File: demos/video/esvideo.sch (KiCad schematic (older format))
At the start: 29 parts, among them U8 BT253, U9 BT473

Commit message: Update demos
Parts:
- C32, C33, C34, C35, C36, C37, C39, C40, C41: symbol C -> video_schlib:C
- C42, C51, C52: symbol CP -> video_schlib:CP
- L5: symbol INDUCTOR -> video_schlib:INDUCTOR
- R15, R22, R23, R24, R36, R37, R38, R42, R43, R44, R45, R46, R47, R8: symbol R -> video_schlib:R
- U8: symbol BT253 -> video_schlib:BT253
- U9: symbol BT473 -> video_schlib:BT473
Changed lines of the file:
@@
-EESchema Schematic File Version 2
-LIBS:video_schlib
-LIBS:power
+EESchema Schematic File Version 4
 LIBS:video-cache
 EELAYER 26 0
@@
 PCA0
 $Comp
-L GND #PWR0162
+L video_schlib:GND #PWR0162
 U 1 1 33A566EB
 P 9300 7800
@@
 Connection ~ 4350 3100
 $Comp
-L GND #PWR0163
+L video_schlib:GND #PWR0163
 U 1 1 3392D11C
 P 4350 4200
@@
 RED_IN
 $Comp
-L GND #PWR0164
+L video_schlib:GND #PWR0164
 U 1 1 335F5DFC
 P 12050 5050
@@
 $EndComp
 $Comp
-L C C32
+L video_schlib:C C32
 U 1 1 335F5DF2
 P 11800 5050
@@
 	6650 4600 6550 4600
 $Comp
-L GND #GND0165
+L video_schlib:GND #GND0165
 U 1 1 A458682C
 P 12850 4250
@@
 $EndComp
 $Comp
-L R R8
+L video_schlib:R R8
 U 1 1 A4586827
 P 12550 4250
@@
 PCA[0..2]
 $Comp
-L GND #GND0166
+L video_schlib:GND #GND0166
 U 1 1 32FA0485
 P 5650 8250
@@
 	11350 3650 13450 3650
 $Comp
-L GND #GND0167
+L video_schlib:GND #GND0167
 U 1 1 32F9F3E8
 P 10450 8250
@@
 RDCAD-
 $Comp
-L BT473 U9
+L video_schlib:BT473 U9
 U 1 1 32F9E902
 P 10350 5450
@@
 $EndComp
 $Comp
-L BT253 U8
+L video_schlib:BT253 U8
 U 1 1 32F9E7F1
 P 5500 5200
@@
 	1700 4600 1800 4600
 $Comp
-L R R42
+L video_schlib:R R42
 U 1 1 84DFB9D2
 P 12600 3000
@@
 $EndComp
 $Comp
-L R R43
+L video_schlib:R R43
 U 1 1 84DFB9D7
 P 12900 3000
@@
 $EndComp
 $Comp
-L R R44
+L video_schlib:R R44
 U 1 1 84DFB9DC
 P 13150 3000
@@
 $EndComp
 $Comp
-L C C33
+L video_schlib:C C33
 U 1 1 84DFBA31
 P 9350 2500
@@
 $EndComp
 $Comp
-L C C34
+L video_schlib:C C34
 U 1 1 84DFBA36
 P 11650 2600
@@
 $EndComp
 $Comp
-L CP C42
+L video_schlib:CP C42
 U 1 1 84DFBAEF
 P 12150 2600
@@
 $EndComp
 $Comp
-L C C35
+L video_schlib:C C35
 U 1 1 84DFBB21
 P 11450 3100
@@
 $EndComp
 $Comp
-L GND #GND0168
+L video_schlib:GND #GND0168
 U 1 1 684863B9
 P 9350 2750
@@
 $EndComp
 $Comp
-L GND #GND0169
+L video_schlib:GND #GND0169
 U 1 1 684863BE
 P 9850 2750
@@
 $EndComp
 $Comp
-L GND #GND0170
+L video_schlib:GND #GND0170
 U 1 1 684863C3
 P 12600 2700
@@
 $EndComp
 $Comp
-L GND #GND0171
+L video_schlib:GND #GND0171
 U 1 1 684863C8
 P 12900 2700
@@
 $EndComp
 $Comp
-L GND #GND0172
+L video_schlib:GND #GND0172
 U 1 1 684863CD
 P 13150 2700
@@
 $EndComp
 $Comp
-L GND #GND0173
+L video_schlib:GND #GND0173
 U 1 1 A44C032A
 P 6650 4400
@@
 $EndComp
 $Comp
-L R R47
+L video_schlib:R R47
 U 1 1 A44C0348
 P 2050 5000
@@
 $EndComp
 $Comp
-L R R45
+L video_schlib:R R45
 U 1 1 A44C032F
 P 2050 5800
@@
 $EndComp
 $Comp
-L R R46
+L video_schlib:R R46
 U 1 1 A44C0339
 P 2050 6600
@@
 $EndComp
 $Comp
-L GND #GND0174
+L video_schlib:GND #GND0174
 U 1 1 A44C0393
 P 2350 5000
@@
 $EndComp
 $Comp
-L GND #GND0175
+L video_schlib:GND #GND0175
 U 1 1 A44C0398
 P 2350 5800
@@
 $EndComp
 $Comp
-L GND #GND0176
+L video_schlib:GND #GND0176
 U 1 1 A44C039D
 P 2350 6600
@@
 $EndComp
 $Comp
-L R R38
+L video_schlib:R R38
 U 1 1 A44C03AC
 P 4100 2900
@@
 $EndComp
 $Comp
-L GND #GND0177
+L video_schlib:GND #GND0177
 U 1 1 A44C03B1
 P 3800 2900
@@
 $EndComp
 $Comp
-L GND #GND0178
+L video_schlib:GND #GND0178
 U 1 1 A44D982F
 P 3800 1450
@@
 $EndComp
 $Comp
-L R R15
+L video_schlib:R R15
 U 1 1 A44D982A
 P 3800 1750
@@
 $EndComp
 $Comp
-L GND #GND0179
+L video_schlib:GND #GND0179
 U 1 1 A44D9852
 P 3300 2800
@@
 $EndComp
 $Comp
-L C C36
+L video_schlib:C C36
 U 1 1 A44D9848
 P 3800 2400
@@
 $EndComp
 $Comp
-L R R36
+L video_schlib:R R36
 U 1 1 A44D9843
 P 4100 2800
@@
 $EndComp
 $Comp
-L C C37
+L video_schlib:C C37
 U 1 1 A44D984D
 P 3550 2800
@@
 $EndComp
 $Comp
-L R R24
+L video_schlib:R R24
 U 1 1 A44C034D
 P 2050 4600
@@
 $EndComp
 $Comp
-L R R23
+L video_schlib:R R23
 U 1 1 A44C0343
 P 2050 5400
@@
 $EndComp
 $Comp
-L R R22
+L video_schlib:R R22
 U 1 1 A44C0334
 P 2050 6200
@@
 $EndComp
 $Comp
-L C C39
+L video_schlib:C C39
 U 1 1 A44C037F
 P 2550 4600
@@
 $EndComp
 $Comp
-L C C40
+L video_schlib:C C40
 U 1 1 A44C0384
 P 2550 5400
@@
 $EndComp
 $Comp
-L C C41
+L video_schlib:C C41
 U 1 1 A44C0389
 P 2550 6200
@@
 $EndComp
 $Comp
-L GND #GND0180
+L video_schlib:GND #GND0180
 U 1 1 26FC0C80
 P 6400 2200
@@
 $EndComp
 $Comp
-L CP C52
+L video_schlib:CP C52
 U 1 1 84DFB9B9
 P 6150 2200
@@
 $EndComp
 $Comp
-L CP C51
+L video_schlib:CP C51
 U 1 1 28ED6A43
 P 9850 2500
@@
 $EndComp
 $Comp
-L INDUCTOR L5
+L video_schlib:INDUCTOR L5
 U 1 1 84DFBB99
 P 12150 1800
@@
 $EndComp
 $Comp
-L R R37
+L video_schlib:R R37
 U 1 1 5D7688E4
 P 3700 3100
@@
 $EndComp
 $Comp
-L GND #GND0181
+L video_schlib:GND #GND0181
 U 1 1 5D7688FD
 P 3400 3100
@@
 REF+
 $Comp
-L VCC #VCC0182
+L video_schlib:VCC #VCC0182
 U 1 1 4BF036B4
 P 12150 1450

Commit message: Update demo to use V5 libs
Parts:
- C32, C33, C34, C35, C36, C37, C52, R15, R22, R23, R24, R36, R37, R38, R42, R43, R44, R45, R46, R47, R8: footprint lib_smd:SM1206 -> Resistor_SMD:R_1206_3216Metric_Pad1.24x1.80mm_HandSolder
- C39, C40, C41, C42, C51: footprint lib_smd:SM1210L -> Resistor_SMD:R_1210_3225Metric_Pad1.24x2.70mm_HandSolder
- L5: footprint lib_smd:SM1812 -> Resistor_SMD:R_1812_4532Metric_Pad1.24x3.50mm_HandSolder
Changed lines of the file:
@@
 F 0 "C32" V 11650 5050 50  0000 C CNN
 F 1 "100nF" V 11950 5050 50  0000 C CNN
-F 2 "lib_smd:SM1206" H 11800 5050 60  0001 C CNN
+F 2 "Resistor_SMD:R_1206_3216Metric_Pad1.24x1.80mm_HandSolder" H 11800 5050 60  0001 C CNN
 F 3 "" H 11800 5050 60  0001 C CNN
 	1    11800 5050
@@
 F 0 "R8" V 12630 4250 50  0000 C CNN
 F 1 "150" V 12550 4250 50  0000 C CNN
-F 2 "lib_smd:SM1206" H 12550 4250 60  0001 C CNN
+F 2 "Resistor_SMD:R_1206_3216Metric_Pad1.24x1.80mm_HandSolder" H 12550 4250 60  0001 C CNN
 F 3 "" H 12550 4250 60  0001 C CNN
 	1    12550 4250
@@
 F 0 "R42" H 12500 3200 50  0000 C CNN
 F 1 "75" V 12600 3000 50  0000 C CNN
-F 2 "lib_smd:SM1206" H 12600 3000 60  0001 C CNN
+F 2 "Resistor_SMD:R_1206_3216Metric_Pad1.24x1.80mm_HandSolder" H 12600 3000 60  0001 C CNN
 F 3 "" H 12600 3000 60  0001 C CNN
 	1    12600 3000
@@
 F 0 "R43" H 12800 3200 50  0000 C CNN
 F 1 "75" V 12900 3000 50  0000 C CNN
-F 2 "lib_smd:SM1206" H 12900 3000 60  0001 C CNN
+F 2 "Resistor_SMD:R_1206_3216Metric_Pad1.24x1.80mm_HandSolder" H 12900 3000 60  0001 C CNN
 F 3 "" H 12900 3000 60  0001 C CNN
 	1    12900 3000
@@
 F 0 "R44" H 13050 3200 50  0000 C CNN
 F 1 "75" V 13150 3000 50  0000 C CNN
-F 2 "lib_smd:SM1206" H 13150 3000 60  0001 C CNN
+F 2 "Resistor_SMD:R_1206_3216Metric_Pad1.24x1.80mm_HandSolder" H 13150 3000 60  0001 C CNN
 F 3 "" H 13150 3000 60  0001 C CNN
 	1    13150 3000
@@
 F 0 "C33" H 9500 2600 50  0000 C CNN
 F 1 "100nF" H 9500 2400 50  0000 C CNN
-F 2 "lib_smd:SM1206" H 9350 2500 60  0001 C CNN
+F 2 "Resistor_SMD:R_1206_3216Metric_Pad1.24x1.80mm_HandSolder" H 9350 2500 60  0001 C CNN
 F 3 "" H 9350 2500 60  0001 C CNN
 	1    9350 2500
@@
 F 0 "C34" H 11800 2700 50  0000 C CNN
 F 1 "100nF" H 11800 2500 50  0000 C CNN
-F 2 "lib_smd:SM1206" H 11650 2600 60  0001 C CNN
+F 2 "Resistor_SMD:R_1206_3216Metric_Pad1.24x1.80mm_HandSolder" H 11650 2600 60  0001 C CNN
 F 3 "" H 11650 2600 60  0001 C CNN
 	1    11650 2600
@@
 F 0 "C42" H 12300 2700 50  0000 C CNN
 F 1 "2.2uF" H 12300 2500 50  0000 C CNN
-F 2 "lib_smd:SM1210L" H 12150 2600 60  0001 C CNN
+F 2 "Resistor_SMD:R_1210_3225Metric_Pad1.24x2.70mm_HandSolder" H 12150 2600 60  0001 C CNN
 F 3 "" H 12150 2600 60  0001 C CNN
 	1    12150 2600
@@
 F 0 "C35" H 11600 3200 50  0000 C CNN
 F 1 "100nF" H 11600 3000 50  0000 C CNN
-F 2 "lib_smd:SM1206" H 11450 3100 60  0001 C CNN
+F 2 "Resistor_SMD:R_1206_3216Metric_Pad1.24x1.80mm_HandSolder" H 11450 3100 60  0001 C CNN
 F 3 "" H 11450 3100 60  0001 C CNN
 	1    11450 3100
@@
 F 0 "R47" V 2130 5000 50  0000 C CNN
 F 1 "75" V 2050 5000 50  0000 C CNN
-F 2 "lib_smd:SM1206" H 2050 5000 60  0001 C CNN
+F 2 "Resistor_SMD:R_1206_3216Metric_Pad1.24x1.80mm_HandSolder" H 2050 5000 60  0001 C CNN
 F 3 "" H 2050 5000 60  0001 C CNN
 	1    2050 5000
@@
 F 0 "R45" V 2130 5800 50  0000 C CNN
 F 1 "75" V 2050 5800 50  0000 C CNN
-F 2 "lib_smd:SM1206" H 2050 5800 60  0001 C CNN
+F 2 "Resistor_SMD:R_1206_3216Metric_Pad1.24x1.80mm_HandSolder" H 2050 5800 60  0001 C CNN
 F 3 "" H 2050 5800 60  0001 C CNN
 	1    2050 5800
@@
 F 0 "R46" V 2130 6600 50  0000 C CNN
 F 1 "75" V 2050 6600 50  0000 C CNN
-F 2 "lib_smd:SM1206" H 2050 6600 60  0001 C CNN
+F 2 "Resistor_SMD:R_1206_3216Metric_Pad1.24x1.80mm_HandSolder" H 2050 6600 60  0001 C CNN
 F 3 "" H 2050 6600 60  0001 C CNN
 	1    2050 6600
@@
 F 0 "R38" V 4180 2900 50  0000 C CNN
 F 1 "510" V 4100 2900 50  0000 C CNN
-F 2 "lib_smd:SM1206" H 4100 2900 60  0001 C CNN
+F 2 "Resistor_SMD:R_1206_3216Metric_Pad1.24x1.80mm_HandSolder" H 4100 2900 60  0001 C CNN
 F 3 "" H 4100 2900 60  0001 C CNN
 	1    4100 2900
@@
 F 0 "R15" V 3880 1750 50  0000 C CNN
 F 1 "1M" V 3800 1750 50  0000 C CNN
-F 2 "lib_smd:SM1206" H 3800 1750 60  0001 C CNN
+F 2 "Resistor_SMD:R_1206_3216Metric_Pad1.24x1.80mm_HandSolder" H 3800 1750 60  0001 C CNN
 F 3 "" H 3800 1750 60  0001 C CNN
 	1    3800 1750
@@
 F 0 "C36" H 3950 2500 50  0000 C CNN
 F 1 "100nF" H 3950 2300 50  0000 C CNN
-F 2 "lib_smd:SM1206" H 3800 2400 60  0001 C CNN
+F 2 "Resistor_SMD:R_1206_3216Metric_Pad1.24x1.80mm_HandSolder" H 3800 2400 60  0001 C CNN
 F 3 "" H 3800 2400 60  0001 C CNN
 	1    3800 2400
@@
 F 0 "R36" V 4180 2800 50  0000 C CNN
 F 1 "470" V 4100 2800 50  0000 C CNN
-F 2 "lib_smd:SM1206" H 4100 2800 60  0001 C CNN
+F 2 "Resistor_SMD:R_1206_3216Metric_Pad1.24x1.80mm_HandSolder" H 4100 2800 60  0001 C CNN
 F 3 "" H 4100 2800 60  0001 C CNN
 	1    4100 2800
@@
 F 0 "C37" V 3800 2800 50  0000 C CNN
 F 1 "100pF" V 3700 2800 50  0000 C CNN
-F 2 "lib_smd:SM1206" H 3550 2800 60  0001 C CNN
+F 2 "Resistor_SMD:R_1206_3216Metric_Pad1.24x1.80mm_HandSolder" H 3550 2800 60  0001 C CNN
 F 3 "" H 3550 2800 60  0001 C CNN
 	1    3550 2800
@@
 F 0 "R24" V 2130 4600 50  0000 C CNN
 F 1 "220" V 2050 4600 50  0000 C CNN
-F 2 "lib_smd:SM1206" H 2050 4600 60  0001 C CNN
+F 2 "Resistor_SMD:R_1206_3216Metric_Pad1.24x1.80mm_HandSolder" H 2050 4600 60  0001 C CNN
 F 3 "" H 2050 4600 60  0001 C CNN
 	1    2050 4600
@@
 F 0 "R23" V 2130 5400 50  0000 C CNN
 F 1 "220" V 2050 5400 50  0000 C CNN
-F 2 "lib_smd:SM1206" H 2050 5400 60  0001 C CNN
+F 2 "Resistor_SMD:R_1206_3216Metric_Pad1.24x1.80mm_HandSolder" H 2050 5400 60  0001 C CNN
 F 3 "" H 2050 5400 60  0001 C CNN
 	1    2050 5400
@@
 F 0 "R22" V 2130 6200 50  0000 C CNN
 F 1 "220" V 2050 6200 50  0000 C CNN
-F 2 "lib_smd:SM1206" H 2050 6200 60  0001 C CNN
+F 2 "Resistor_SMD:R_1206_3216Metric_Pad1.24x1.80mm_HandSolder" H 2050 6200 60  0001 C CNN
 F 3 "" H 2050 6200 60  0001 C CNN
 	1    2050 6200
@@
 F 0 "C39" V 2400 4600 50  0000 C CNN
 F 1 "1uF" V 2700 4600 50  0000 C CNN
-F 2 "lib_smd:SM1210L" H 2550 4600 60  0001 C CNN
+F 2 "Resistor_SMD:R_1210_3225Metric_Pad1.24x2.70mm_HandSolder" H 2550 4600 60  0001 C CNN
 F 3 "" H 2550 4600 60  0001 C CNN
 	1    2550 4600
@@
 F 0 "C40" V 2400 5400 50  0000 C CNN
 F 1 "1uF" V 2700 5400 50  0000 C CNN
-F 2 "lib_smd:SM1210L" H 2550 5400 60  0001 C CNN
+F 2 "Resistor_SMD:R_1210_3225Metric_Pad1.24x2.70mm_HandSolder" H 2550 5400 60  0001 C CNN
 F 3 "" H 2550 5400 60  0001 C CNN
 	1    2550 5400
@@
 F 0 "C41" V 2400 6200 50  0000 C CNN
 F 1 "1uF" V 2700 6200 50  0000 C CNN
-F 2 "lib_smd:SM1210L" H 2550 6200 60  0001 C CNN
+F 2 "Resistor_SMD:R_1210_3225Metric_Pad1.24x2.70mm_HandSolder" H 2550 6200 60  0001 C CNN
 F 3 "" H 2550 6200 60  0001 C CNN
 	1    2550 6200
@@
 F 0 "C52" V 6300 2200 50  0000 C CNN
 F 1 "22uF" V 6000 2200 50  0000 C CNN
-F 2 "lib_smd:SM1206" H 6150 2200 60  0001 C CNN
+F 2 "Resistor_SMD:R_1206_3216Metric_Pad1.24x1.80mm_HandSolder" H 6150 2200 60  0001 C CNN
 F 3 "" H 6150 2200 60  0001 C CNN
 	1    6150 2200
@@
 F 0 "C51" H 10000 2600 50  0000 C CNN
 F 1 "22uF" H 10000 2400 50  0000 C CNN
-F 2 "lib_smd:SM1210L" H 9850 2500 60  0001 C CNN
+F 2 "Resistor_SMD:R_1210_3225Metric_Pad1.24x2.70mm_HandSolder" H 9850 2500 60  0001 C CNN
 F 3 "" H 9850 2500 60  0001 C CNN
 	1    9850 2500
@@
 F 0 "L5" H 12350 1850 50  0000 C CNN
 F 1 "22uH" H 12350 1750 50  0000 C CNN
-F 2 "lib_smd:SM1812" H 12150 1800 60  0001 C CNN
+F 2 "Resistor_SMD:R_1812_4532Metric_Pad1.24x3.50mm_HandSolder" H 12150 1800 60  0001 C CNN
 F 3 "" H 12150 1800 60  0001 C CNN
 	1    12150 1800
@@
 F 0 "R37" V 3780 3100 50  0000 C CNN
 F 1 "510" V 3700 3100 50  0000 C CNN
-F 2 "lib_smd:SM1206" H 3700 3100 60  0001 C CNN
+F 2 "Resistor_SMD:R_1206_3216Metric_Pad1.24x1.80mm_HandSolder" H 3700 3100 60  0001 C CNN
 F 3 "" H 3700 3100 60  0001 C CNN
 	1    3700 3100

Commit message: Update demo "video" to use V5 libraries
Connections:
- wire segments 184 -> 225
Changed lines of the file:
@@
 EESchema Schematic File Version 4
 LIBS:video-cache
-EELAYER 26 0
+EELAYER 29 0
 EELAYER END
 $Descr A3 16535 11693
@@
 	4450 3200 4350 3200
 Wire Wire Line
-	4350 3100 4350 3800
+	4350 3100 4350 3200
 Wire Wire Line
 	4350 3800 4450 3800
@@
 Connection ~ 11500 5050
 Wire Wire Line
-	11350 5050 11600 5050
+	11350 5050 11500 5050
 Wire Wire Line
 	11500 5050 11500 4450
@@
 	11450 4850 11350 4850
 Wire Wire Line
-	11450 3300 11450 4850
+	11450 3300 11450 4650
 Wire Wire Line
 	9350 7550 8950 7550
@@
 Connection ~ 12150 4250
 Wire Wire Line
-	11350 4250 12300 4250
-Wire Wire Line
-	12150 2800 12150 4250
+	11350 4250 12150 4250
+Wire Wire Line
+	12150 2800 12150 2900
 Wire Wire Line
 	11450 4650 11350 4650
@@
 	13150 3850 13150 3250
 Wire Wire Line
-	11350 3850 13450 3850
+	11350 3850 13150 3850
 Wire Wire Line
 	12900 3650 12900 3250
 Wire Wire Line
-	11350 3650 13450 3650
+	11350 3650 12900 3650
 $Comp
 L video_schlib:GND #GND0167
@@
 $EndComp
 Wire Wire Line
-	1700 6200 1800 6200
+	1700 6200 1750 6200
 Wire Wire Line
 	3800 2100 4450 2100
@@
 Connection ~ 6550 4700
 Wire Wire Line
-	6550 4600 6550 4800
+	6550 4600 6550 4700
 Wire Wire Line
 	6550 3700 6550 3800
@@
 Connection ~ 6550 4300
 Wire Wire Line
-	6550 4200 6550 4400
+	6550 4200 6550 4300
 Wire Wire Line
 	6550 4400 6650 4400
@@
 Connection ~ 4450 3900
 Wire Wire Line
-	4450 4200 4450 4400
-Wire Wire Line
-	4450 3800 4450 4000
+	4450 4200 4450 4300
+Wire Wire Line
+	4450 3800 4450 3900
 Text HLabel 9300 7250 0    60   Input ~ 0
 WRCDA-
@@
 $EndComp
 Wire Wire Line
-	3800 2000 3800 2200
+	3800 2000 3800 2100
 Wire Wire Line
 	3800 2800 3800 2600
 Wire Wire Line
-	3750 2800 3850 2800
+	3750 2800 3800 2800
 Wire Wire Line
 	2750 6200 3000 6200
@@
 	2750 4600 4450 4600
 Wire Wire Line
-	1700 5400 1800 5400
-Wire Wire Line
-	1700 4600 1800 4600
+	1700 5400 1750 5400
+Wire Wire Line
+	1700 4600 1750 4600
 $Comp
 L video_schlib:R R42
@@
 Connection ~ 13150 3850
 Wire Wire Line
-	5350 2200 5950 2200
-Wire Wire Line
-	9350 2200 12150 2200
-Wire Wire Line
-	10050 2750 10550 2750
-Wire Wire Line
-	11350 3450 13450 3450
-Wire Wire Line
-	3950 3100 4450 3100
+	5350 2200 5450 2200
+Wire Wire Line
+	9350 2200 9850 2200
+Wire Wire Line
+	10050 2750 10150 2750
+Wire Wire Line
+	11350 3450 12600 3450
+Wire Wire Line
+	3950 3100 4350 3100
 Wire Wire Line
 	4450 4700 2900 4700
@@
 Connection ~ 6550 4000
 Wire Wire Line
-	12150 2100 12150 2400
+	12150 2100 12150 2200
 Connection ~ 12150 2200
 Wire Wire Line
@@
 	11400 5850 11350 5850
 Wire Wire Line
-	10450 8150 10450 8250
-Wire Wire Line
-	10150 8200 10450 8200
+	10450 8150 10450 8200
+Wire Wire Line
+	10150 8200 10250 8200
 Wire Wire Line
 	10350 8200 10350 8150
@@
 Connection ~ 10250 8200
 Wire Wire Line
-	9300 7650 9300 7800
+	9300 7650 9300 7750
 Wire Wire Line
 	9300 7650 9350 7650
@@
 	9350 7250 9300 7250
 Wire Wire Line
-	5650 8100 5650 8250
-Wire Wire Line
-	5350 8150 5650 8150
+	5650 8100 5650 8150
+Wire Wire Line
+	5350 8150 5450 8150
 Wire Wire Line
 	5350 8150 5350 8100
@@
 Wire Wire Line
 	12150 1450 12150 1500
+Wire Wire Line
+	4350 3100 4450 3100
+Wire Wire Line
+	4350 3600 4350 3800
+Wire Wire Line
+	4350 3500 4350 3600
+Wire Wire Line
+	4350 3400 4350 3500
+Wire Wire Line
+	4350 3300 4350 3400
+Wire Wire Line
+	4350 3200 4350 3300
+Wire Wire Line
+	11450 4650 11450 4850
+Wire Wire Line
+	11500 5050 11600 5050
+Wire Wire Line
+	12150 4250 12300 4250
+Wire Wire Line
+	6550 4700 6550 4800
+Wire Wire Line
+	6550 4300 6550 4400
+Wire Wire Line
+	4450 4300 4450 4400
+Wire Wire Line
+	4450 3900 4450 4000
+Wire Wire Line
+	10250 2750 10350 2750
+Wire Wire Line
+	10150 2750 10250 2750
+Wire Wire Line
+	9850 2200 10550 2200
+Wire Wire Line
+	10550 2200 11450 2200
+Wire Wire Line
+	11450 2200 11650 2200
+Wire Wire Line
+	11650 2200 12150 2200
+Wire Wire Line
+	10350 2750 10450 2750
+Wire Wire Line
+	10450 2750 10550 2750
+Wire Wire Line
+	12600 3450 13450 3450
+Wire Wire Line
+	12900 3650 13450 3650
+Wire Wire Line
+	13150 3850 13450 3850
+Wire Wire Line
+	1750 5400 1800 5400
+Wire Wire Line
+	1750 6200 1800 6200
+Wire Wire Line
+	1750 4600 1800 4600
+Wire Wire Line
+	3800 2100 3800 2200
+Wire Wire Line
+	3800 2800 3850 2800
+Wire Wire Line
+	12150 2200 12150 2400
+Wire Wire Line
+	12150 2900 12150 4250
+Wire Wire Line
+	10450 8200 10450 8250
+Wire Wire Line
+	10350 8200 10450 8200
+Wire Wire Line
+	10250 8200 10350 8200
+Wire Wire Line
+	9300 7750 9300 7800
+Wire Wire Line
+	5650 8150 5650 8250
+Wire Wire Line
+	5450 8150 5550 8150
+Wire Wire Line
+	5550 8150 5650 8150
+Wire Wire Line
+	5650 2200 5950 2200
+Wire Wire Line
+	5550 2200 5650 2200
+Wire Wire Line
+	5450 2200 5550 2200
 $EndSCHEMATC

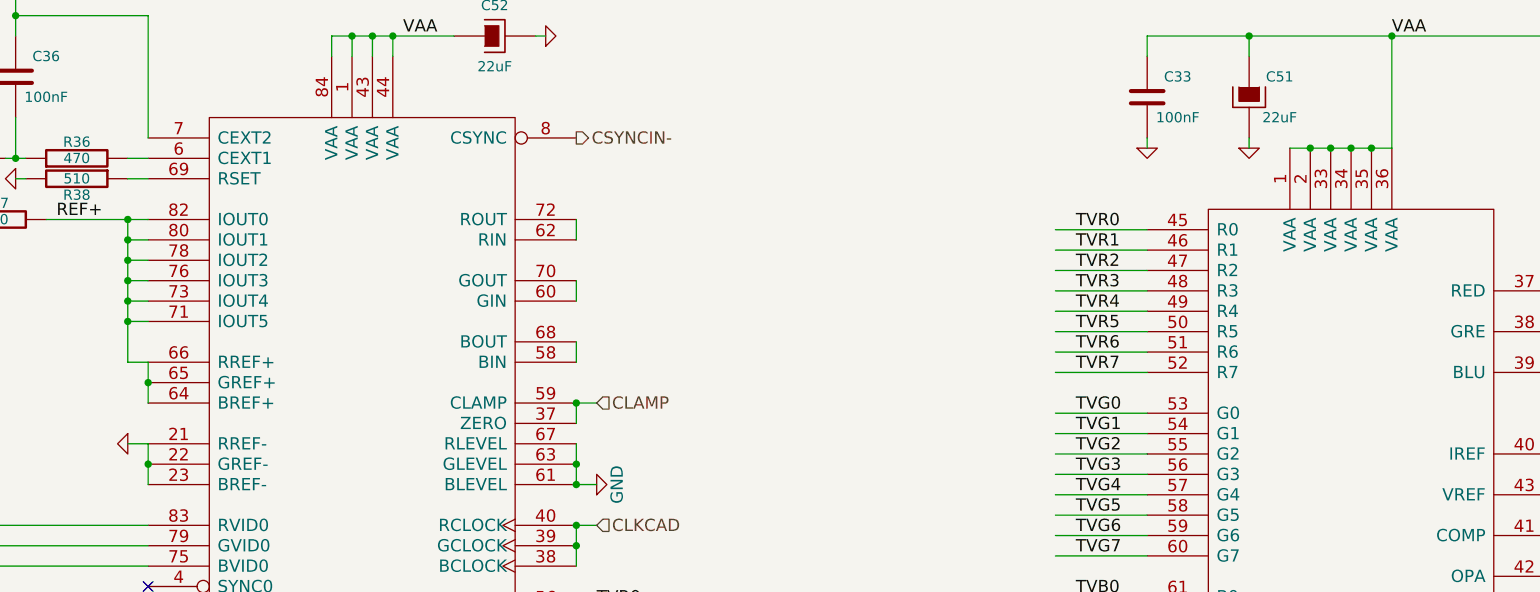
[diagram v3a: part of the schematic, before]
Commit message: Update demo "video"
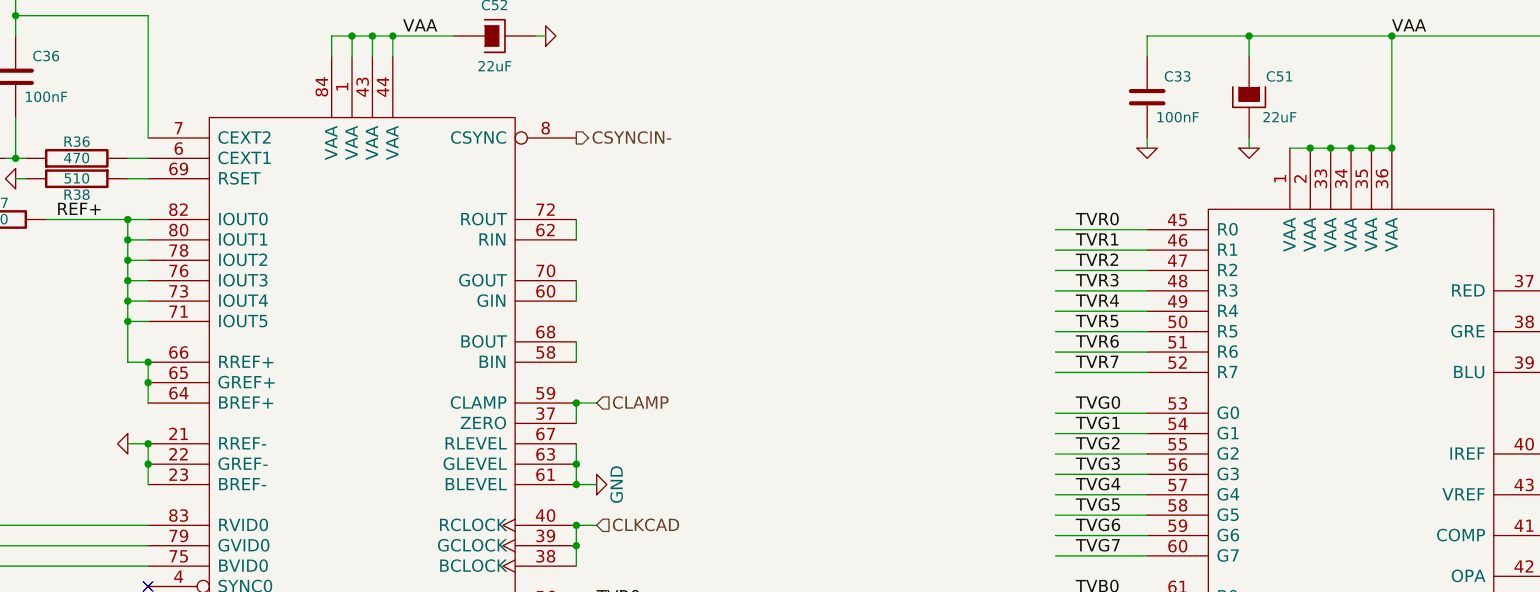
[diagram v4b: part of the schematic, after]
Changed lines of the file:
@@
-EESchema Schematic File Version 4
+EESchema Schematic File Version 5
 LIBS:video-cache
-EELAYER 29 0
+EELAYER 30 0
 EELAYER END
 $Descr A3 16535 11693
@@
 Wire Wire Line
 	5450 2200 5550 2200
+Connection ~ 10550 2750
+Connection ~ 4450 4200
+Connection ~ 4450 3800
 $EndSCHEMATC
